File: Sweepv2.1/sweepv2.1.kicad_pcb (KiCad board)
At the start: 2 copper layers, 216.9 x 86.9 mm, 51 parts, among them J1 AudioJack4dpb, J2 AudioJack4dpb, SW10 SW_Push, SW11 SW_Push, SW11_r1 SW_Push, SW12 SW_Push, SW12_r1 SW_Push, SW13_r1 SW_Push, SW14 SW_Push, SW15 SW_Push, SW15_r1 SW_Push, SW16 SW_Push, SW16_r1 SW_Push, SW17 SW_Push, SW17_r1 SW_Push, SW18 SW_Push, SW18_r1 SW_Push, SW2 SW_Push, SW20 SW_Push, SW20_r1 SW_Push, SW21 SW_Push, SW21_r1 SW_Push, SW2_r1 SW_Push, SW3 SW_Push, SW3_r1 SW_Push, SW4 SW_Push, SW4_r1 SW_Push, SW5 SW_Push, SW5_r1 SW_Push, SW6 SW_Push, SW6_r1 SW_Push, SW7_r1 SW_Push, SW8 SW_Push, SW8_r1 SW_Push, SW9 SW_Push, SW9_r1 SW_Push, U1 ProMicro-kbd, U2 ProMicro-kbd

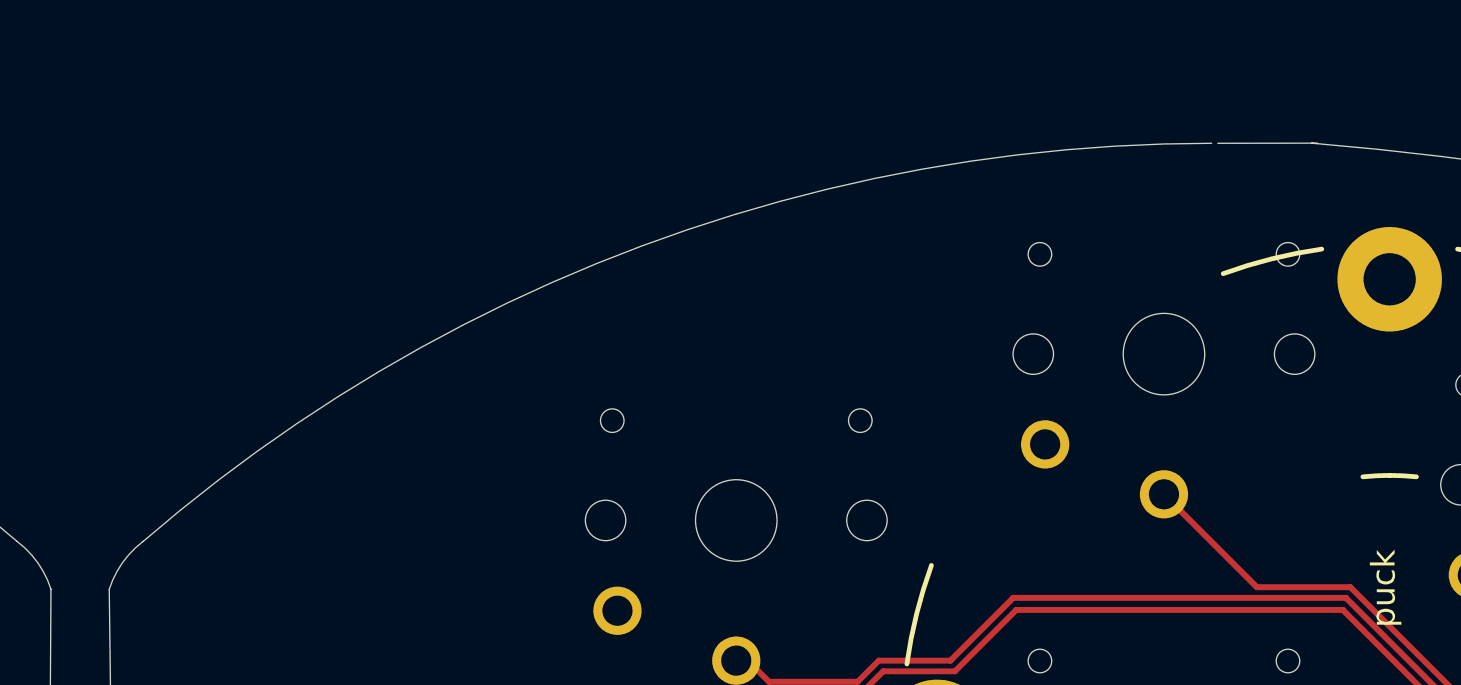
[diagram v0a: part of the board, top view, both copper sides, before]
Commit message: Add gerbers
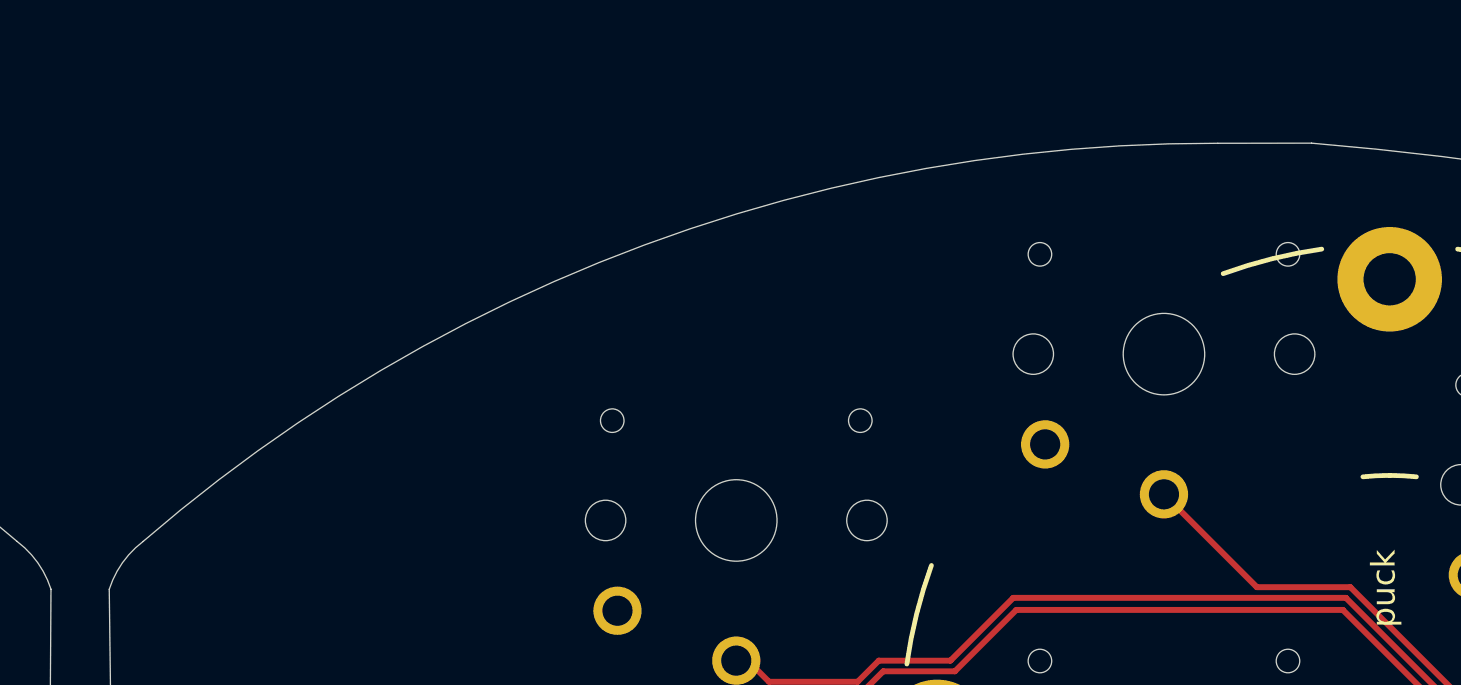
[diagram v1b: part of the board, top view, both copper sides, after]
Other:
- outline, holes or cut-outs redrawn
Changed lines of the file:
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@@
   (gr_line (start 128.96 77.724) (end 128.975507 89.545022) (layer Edge.Cuts) (width 0.05))
   (gr_arc (start 22.542 50.442) (end 21.792 50.442) (angle 90) (layer Edge.Cuts) (width 0.05))
-  (gr_line (start 182.321777 21.502679) (end 178.120389 21.508139) (layer Edge.Cuts) (width 0.05))
+  (gr_line (start 182.067777 21.502679) (end 178.120389 21.508139) (layer Edge.Cuts) (width 0.05))
   (gr_arc (start 221.926148 81.404051) (end 236.953304 88.85815) (angle -25.93947102) (layer Edge.Cuts) (width 0.05))
   (gr_line (start 236.953304 88.85815) (end 226.446 107.451265) (layer Edge.Cuts) (width 0.05))
-  (gr_arc (start 177.866389 90.238139) (end 177.866389 21.508139) (angle -40.87028694) (layer Edge.Cuts) (width 0.05))
+  (gr_arc (start 177.866389 90.238139) (end 178.120389 21.508139) (angle -41.08203009) (layer Edge.Cuts) (width 0.05))
   (gr_line (start 222.033002 49.694917) (end 237.938 49.692) (layer Edge.Cuts) (width 0.05))
   (gr_line (start 219.998001 47.763999) (end 219.998045 30.439419) (layer Edge.Cuts) (width 0.05))
